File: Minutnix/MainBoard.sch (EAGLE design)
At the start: 31 parts, among them IC1 MEGA8-AI, IC2 74LS47N, IC3 74LS47N

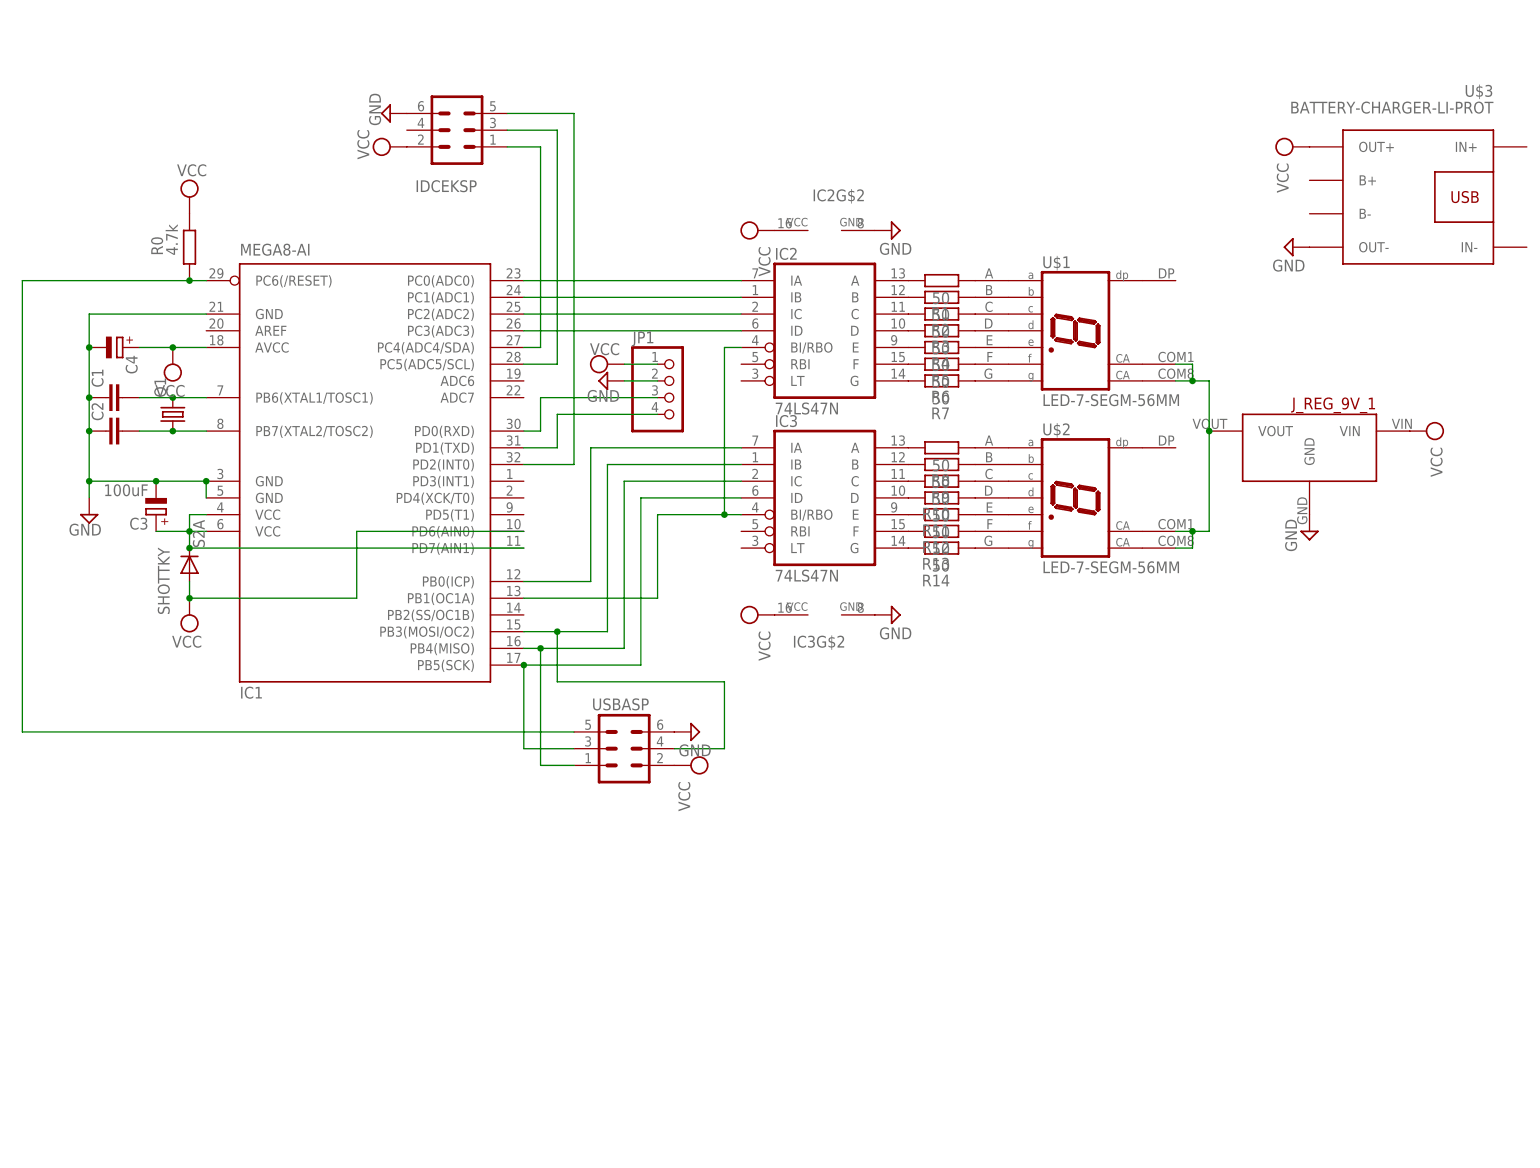
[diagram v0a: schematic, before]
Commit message: Wersja 1
Do kubełka 1
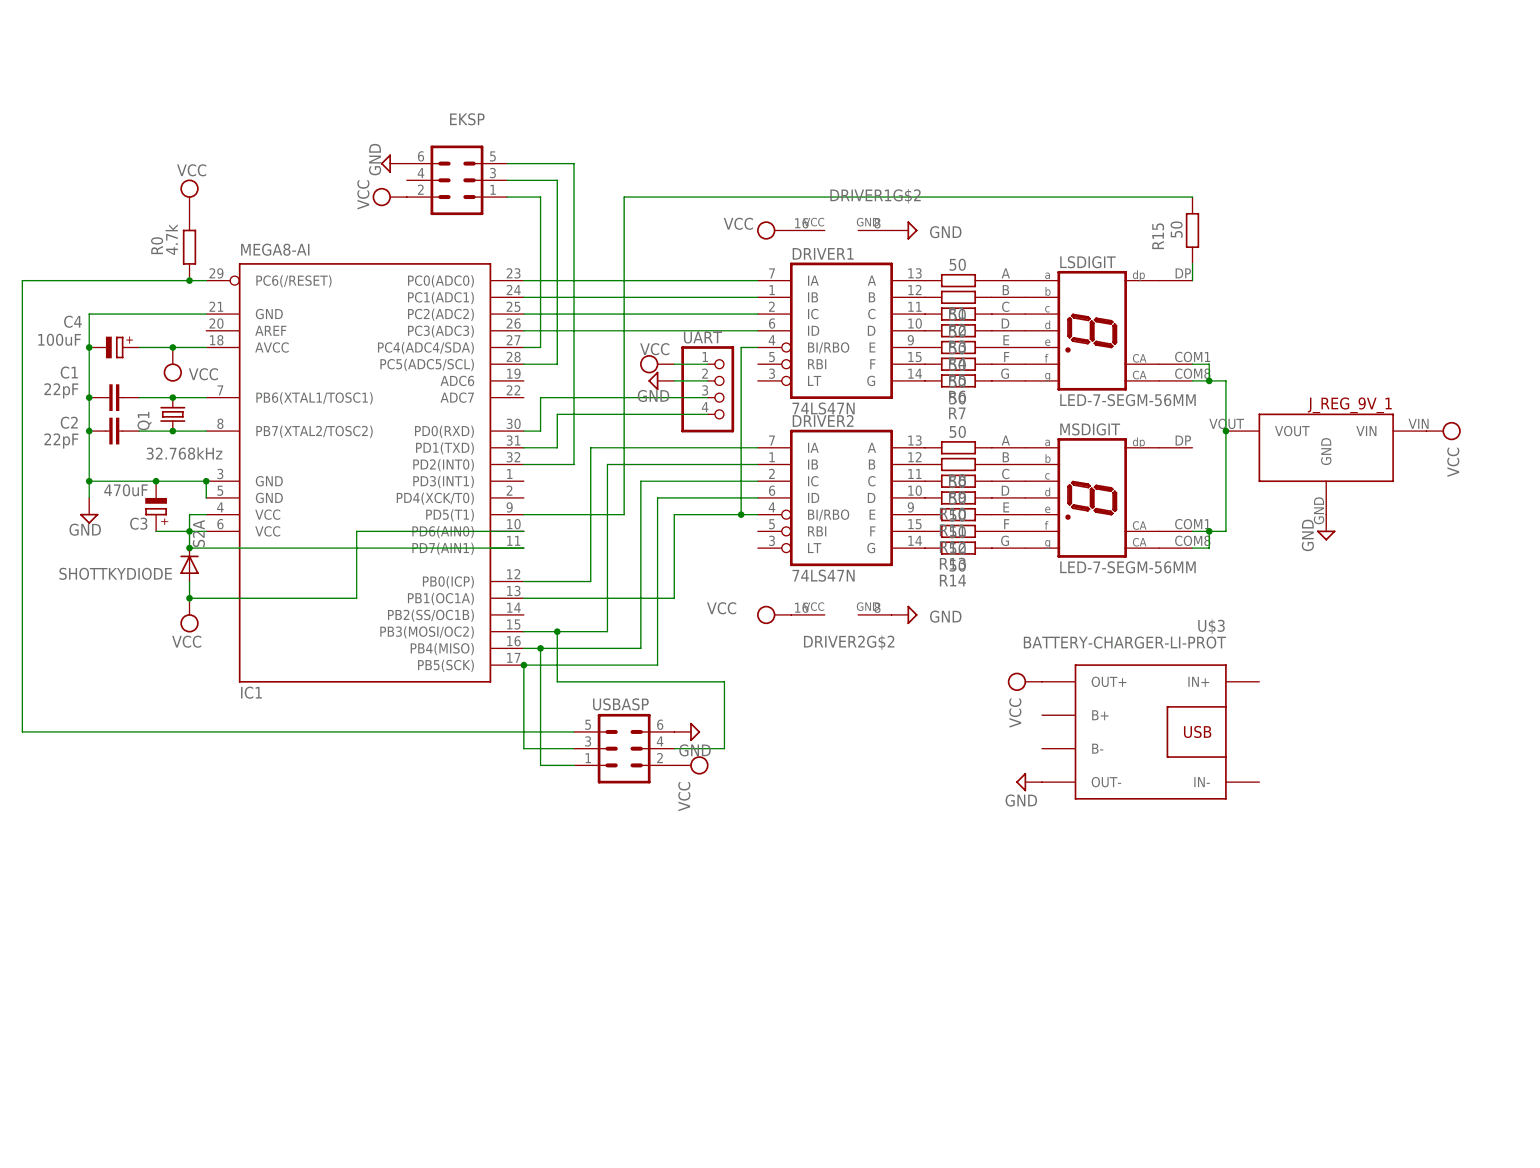
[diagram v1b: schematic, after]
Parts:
- removed IC2, IC3: 74LS47N, 74xx-eu:74LS47N
- removed IDCEKSP: (no value), con-harting-ml:ML6
- removed JP1: (no value), pinhead:PINHD-1X4
- removed U$1, U$2: LED-7-SEGM-56MM, BigLED7Segm:LED-7-SEGM-56MM
- added DRIVER1, DRIVER2: 74LS47N, 74xx-eu:74LS47N
- added EKSP: (no value), con-harting-ml:ML6
- added LSDIGIT, MSDIGIT: LED-7-SEGM-56MM, BigLED7Segm:LED-7-SEGM-56MM
- added R15: 50, rcl:R-EU_01005
- added UART: (no value), pinhead:PINHD-1X4
- C1, C2: value (none) -> 22pF
- C3: value 100uF -> 470uF
- C4: value (none) -> 100uF
- Q1: value (none) -> 32.768kHz
- renumbered SHOTTKY to SHOTTKYDIODE
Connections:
- new net N$32: LSDIGIT.DP, R15.1
- new net N$33: IC1.PD5(T1), R15.2
- net GND: now also DRIVER1G$2.GND, DRIVER2G$2.GND, EKSP.6, UART.2; no longer IC2G$2.GND, IC3G$2.GND, IDCEKSP.6, JP1.2
- net N$10: now also DRIVER1G$1.F; no longer IC2G$1.F
- net N$11: now also DRIVER1G$1.G; no longer IC2G$1.G
- net N$12: now also EKSP.1; no longer IDCEKSP.1
- net N$13: now also LSDIGIT.A; no longer U$1.A
- net N$14: now also EKSP.5; no longer IDCEKSP.5
- net N$15: now also LSDIGIT.B; no longer U$1.B
- net N$16: now also LSDIGIT.C; no longer U$1.C
- net N$17: now also LSDIGIT.D; no longer U$1.D
- net N$18: now also LSDIGIT.E; no longer U$1.E
- net N$19: now also LSDIGIT.F; no longer U$1.F
- net N$20: now also EKSP.3; no longer IDCEKSP.3
- net N$21: now also DRIVER2G$1.ID; no longer IC3G$1.ID
- net N$23: now also DRIVER2G$1.IB; no longer IC3G$1.IB
- net N$24: now also DRIVER2G$1.IC; no longer IC3G$1.IC
- net N$25: now also LSDIGIT.G; no longer U$1.G
- net N$26: now also DRIVER1G$1.IA; no longer IC2G$1.IA
- net N$27: now also DRIVER1G$1.IB; no longer IC2G$1.IB
- net N$28: now also DRIVER1G$1.IC; no longer IC2G$1.IC
- net N$29: now also DRIVER1G$1.ID; no longer IC2G$1.ID
- net N$3: now also DRIVER2G$1.IA; no longer IC3G$1.IA
- net N$30: now also UART.4; no longer JP1.4
- net N$31: now also UART.3; no longer JP1.3
- net N$34: now also MSDIGIT.A; no longer U$2.A
- net N$36: now also LSDIGIT.CA1, LSDIGIT.CA8, MSDIGIT.CA1, MSDIGIT.CA8; no longer U$1.CA1, U$1.CA8, U$2.CA1, U$2.CA8
- net N$37: now also MSDIGIT.B; no longer U$2.B
- net N$38: now also MSDIGIT.C; no longer U$2.C
- net N$39: now also MSDIGIT.D; no longer U$2.D
- net N$4: now also DRIVER1G$1.BI/RBO, DRIVER2G$1.BI/RBO; no longer IC2G$1.BI/RBO, IC3G$1.BI/RBO
- net N$40: now also MSDIGIT.E; no longer U$2.E
- net N$41: now also MSDIGIT.F; no longer U$2.F
- net N$42: now also MSDIGIT.G; no longer U$2.G
- net N$44: now also DRIVER2G$1.G; no longer IC3G$1.G
- net N$45: now also DRIVER2G$1.F; no longer IC3G$1.F
- net N$46: now also DRIVER2G$1.E; no longer IC3G$1.E
- net N$47: now also DRIVER2G$1.D; no longer IC3G$1.D
- net N$48: now also DRIVER2G$1.C; no longer IC3G$1.C
- net N$49: now also DRIVER2G$1.B; no longer IC3G$1.B
- net N$5: now also DRIVER1G$1.A; no longer IC2G$1.A
- net N$50: now also DRIVER2G$1.A; no longer IC3G$1.A
- net N$6: now also DRIVER1G$1.B; no longer IC2G$1.B
- net N$7: now also DRIVER1G$1.C; no longer IC2G$1.C
- net N$8: now also DRIVER1G$1.D; no longer IC2G$1.D
- net N$9: now also DRIVER1G$1.E; no longer IC2G$1.E
- net VCC: now also DRIVER1G$2.VCC, DRIVER2G$2.VCC, EKSP.2, UART.1; no longer IC2G$2.VCC, IC3G$2.VCC, IDCEKSP.2, JP1.1
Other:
- moved on the sheet: J_REG_9V_1, R1, R10, R11, R12, R13, R14, R2, R3, R4, R5, R6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

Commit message: Archivisation and actualisation
Archivisation of 1 version of boards
New version of boards
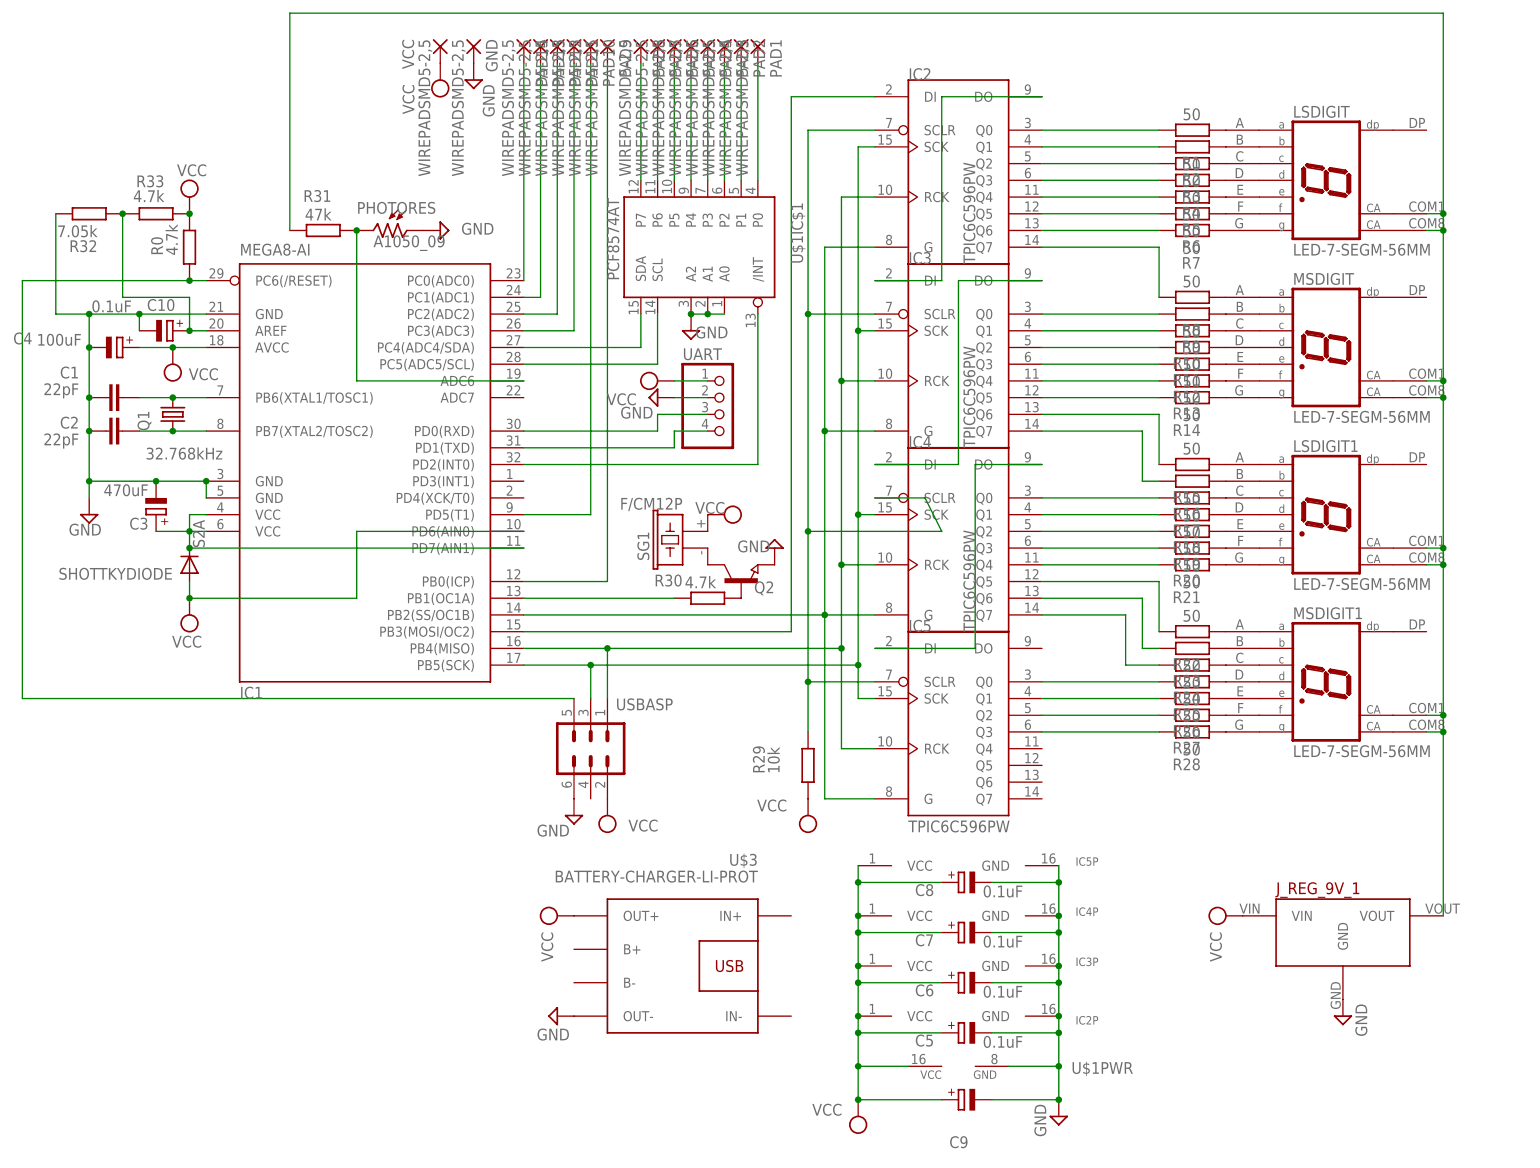
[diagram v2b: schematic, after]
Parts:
- removed DRIVER1, DRIVER2: 74LS47N, 74xx-eu:74LS47N
- removed EKSP: (no value), con-harting-ml:ML6
- added C10, C5, C6, C7, C8: 0.1uF, rcl:CPOL-EU140CLH-1010
- added C9: (no value), rcl:CPOL-EU140CLH-1010
- added GND, PAD1, PAD10, PAD11, PAD12, PAD13, PAD14, PAD2, PAD3, PAD4, PAD5, PAD6, PAD7, PAD8, PAD9, VCC: WIREPADSMD5-2,5, wirepad:WIREPADSMD5-2,5
- added IC2, IC3, IC4, IC5: TPIC6C596PW, tpic:TPIC6C596PW
- added LSDIGIT1, MSDIGIT1: LED-7-SEGM-56MM, BigLED7Segm:LED-7-SEGM-56MM
- added PHOTORES: A1050_09, photo-elements:A1050_09
- added Q2: (no value), semicon-smd-ipc:NPN-TRANSISTOR_SOT23
- added R16, R17, R18, R19, R20, R21, R22, R23, R24, R25, R26, R27, R28: 50, rcl:R-EU_01005
- added R29: 10k, rcl:R-EU_01005
- added R30, R33: 4.7k, rcl:R-EU_01005
- added R31: 47k, rcl:R-EU_01005
- added R32: 7.05k, rcl:R-EU_01005
- added SG1: F/CM12P, buzzer:F/CM12P
- added U$1: PCF8574AT, i2c:PCF8574AT
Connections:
- new net N$43: IC2G$1.Q7, R8.2
- new net N$51: MSDIGIT1.A, R22.1
- new net N$52: MSDIGIT1.B, R23.1
- new net N$53: MSDIGIT1.C, R24.1
- new net N$54: MSDIGIT1.D, R25.1
- new net N$55: MSDIGIT1.E, R26.1
- new net N$56: MSDIGIT1.F, R27.1
- new net N$57: MSDIGIT1.G, R28.1
- new net N$58: IC3G$1.Q0, R9.2
- new net N$59: IC3G$1.Q1, R10.2
- new net N$60: IC3G$1.Q2, R11.2
- new net N$61: IC3G$1.Q3, R12.2
- new net N$62: IC3G$1.Q4, R13.2
- new net N$63: IC3G$1.Q5, R14.2
- new net N$64: IC3G$1.Q6, R15.2
- new net N$65: IC3G$1.Q7, R16.2
- new net N$66: IC4G$1.Q0, R17.2
- new net N$67: IC4G$1.Q1, R18.2
- new net N$68: IC4G$1.Q2, R19.2
- new net N$69: IC4G$1.Q3, R20.2
- new net N$70: IC4G$1.Q4, R21.2
- new net N$71: IC4G$1.Q5, R22.2
- new net N$72: IC4G$1.Q6, R23.2
- new net N$73: IC4G$1.Q7, R24.2
- new net N$74: IC5G$1.Q0, R25.2
- new net N$75: IC5G$1.Q1, R26.2
- new net N$76: IC5G$1.Q2, R27.2
- new net N$77: IC5G$1.Q3, R28.2
- new net N$78: IC3G$1.DO, IC4G$1.DI
- new net N$79: IC4G$1.DO, IC5G$1.DI
- new net N$80: IC2G$1.DO, IC3G$1.DI
- new net N$81: IC1.PC5(ADC5/SCL), U$1IC$1.SCL
- new net N$82: IC1.PC3(ADC3), PAD11.P
- new net N$83: IC1.PB0(ICP), PAD9.P
- new net N$84: IC1.PD5(T1), PAD10.P
- new net N$85: PAD1.P, U$1IC$1.P0
- new net N$86: PAD2.P, U$1IC$1.P1
- new net N$87: PAD3.P, U$1IC$1.P2
- new net N$88: PAD4.P, U$1IC$1.P3
- new net N$89: PAD5.P, U$1IC$1.P4
- new net N$90: PAD6.P, U$1IC$1.P5
- new net N$91: PAD7.P, U$1IC$1.P6
- new net N$92: PAD8.P, U$1IC$1.P7
- new net N$93: IC1.ADC6, PHOTORES.2, R31.1
- net GND: now also C10.-, C5.-, C6.-, C7.-, C8.-, C9.-, GND.P, IC2P.GND, IC3P.GND, IC4P.GND, IC5P.GND, PHOTORES.1, Q2.E, R32.2, U$1IC$1.A0, U$1IC$1.A1, U$1IC$1.A2, U$1PWR.GND; no longer DRIVER1G$2.GND, DRIVER2G$2.GND, EKSP.6
- net N$10: now also IC2G$1.Q5; no longer DRIVER1G$1.F
- net N$11: now also IC2G$1.Q6; no longer DRIVER1G$1.G
- net N$12: now also IC1.PC0(ADC0), PAD14.P; no longer EKSP.1, IC1.PC4(ADC4/SDA)
- net N$14: now also IC1.PC1(ADC1), PAD13.P; no longer EKSP.5, IC1.PD2(INT0)
- net N$20: now also IC1.PC2(ADC2), PAD12.P; no longer EKSP.3, IC1.PC5(ADC5/SCL)
- net N$21: now also Q2.B, R30.1; no longer DRIVER2G$1.ID, IC1.PB5(SCK), USBASP.3
- net N$23: now also IC2G$1.DI; no longer DRIVER2G$1.IB, USBASP.4
- net N$24: now also IC2G$1.SCLR, IC3G$1.SCLR, IC4G$1.SCLR, IC5G$1.SCLR, R29.1; no longer DRIVER2G$1.IC, IC1.PB4(MISO), USBASP.1
- net N$26: now also IC1.PB5(SCK), IC2G$1.SCK, IC3G$1.SCK, IC4G$1.SCK, IC5G$1.SCK, USBASP.3; no longer DRIVER1G$1.IA, IC1.PC0(ADC0)
- net N$27: now also IC1.PB4(MISO), IC2G$1.RCK, IC3G$1.RCK, IC4G$1.RCK, IC5G$1.RCK, USBASP.1; no longer DRIVER1G$1.IB, IC1.PC1(ADC1)
- net N$28: now also J_REG_9V_1.VOUT, LSDIGIT.CA1, LSDIGIT.CA8, LSDIGIT1.CA1, LSDIGIT1.CA8, MSDIGIT.CA1, MSDIGIT.CA8, MSDIGIT1.CA1, MSDIGIT1.CA8, R31.2; no longer DRIVER1G$1.IC, IC1.PC2(ADC2)
- net N$29: now also Q2.C, SG1.2; no longer DRIVER1G$1.ID, IC1.PC3(ADC3)
- net N$3: now also IC1.PB1(OC1A), R30.2; no longer DRIVER2G$1.IA, IC1.PB0(ICP)
- net N$32: now also C10.+, IC1.AREF, R32.1, R33.2; no longer LSDIGIT.DP, R15.1
- net N$33: now also IC1.PC4(ADC4/SDA), U$1IC$1.SDA; no longer IC1.PD5(T1), R15.2
- net N$36: now also IC1.PD2(INT0), U$1IC$1./INT; no longer J_REG_9V_1.VOUT, LSDIGIT.CA1, LSDIGIT.CA8, MSDIGIT.CA1, MSDIGIT.CA8
- net N$4: now also IC1.PB2(SS/OC1B), IC2G$1.G, IC3G$1.G, IC4G$1.G, IC5G$1.G; no longer DRIVER1G$1.BI/RBO, DRIVER2G$1.BI/RBO, IC1.PB1(OC1A)
- net N$44: now also LSDIGIT1.A, R15.1; no longer DRIVER2G$1.G, R14.2
- net N$45: now also LSDIGIT1.B, R16.1; no longer DRIVER2G$1.F, R13.2
- net N$46: now also LSDIGIT1.C, R17.1; no longer DRIVER2G$1.E, R12.2
- net N$47: now also LSDIGIT1.D, R18.1; no longer DRIVER2G$1.D, R11.2
- net N$48: now also LSDIGIT1.E, R19.1; no longer DRIVER2G$1.C, R10.2
- net N$49: now also LSDIGIT1.F, R20.1; no longer DRIVER2G$1.B, R9.2
- net N$5: now also IC2G$1.Q0; no longer DRIVER1G$1.A
- net N$50: now also LSDIGIT1.G, R21.1; no longer DRIVER2G$1.A, R8.2
- net N$6: now also IC2G$1.Q1; no longer DRIVER1G$1.B
- net N$7: now also IC2G$1.Q2; no longer DRIVER1G$1.C
- net N$8: now also IC2G$1.Q3; no longer DRIVER1G$1.D
- net N$9: now also IC2G$1.Q4; no longer DRIVER1G$1.E
- net VCC: now also C5.+, C6.+, C7.+, C8.+, C9.+, IC2P.VCC, IC3P.VCC, IC4P.VCC, IC5P.VCC, R29.2, R33.1, SG1.1, U$1PWR.VCC, VCC.P; no longer DRIVER1G$2.VCC, DRIVER2G$2.VCC, EKSP.2
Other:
- moved on the sheet: J_REG_9V_1, LSDIGIT, MSDIGIT, R1, R10, R11, R12, R13, R14, R15, R2, R3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
